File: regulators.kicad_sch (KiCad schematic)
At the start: 47 parts, among them J6 Screw_Terminal_01x02, J7 Screw_Terminal_01x02, SW2 SKRPANE010, U1 STM32H723ZGT6, U7 AP62300TWU, U8 AP2112K-3.3, Y3 25 MHz

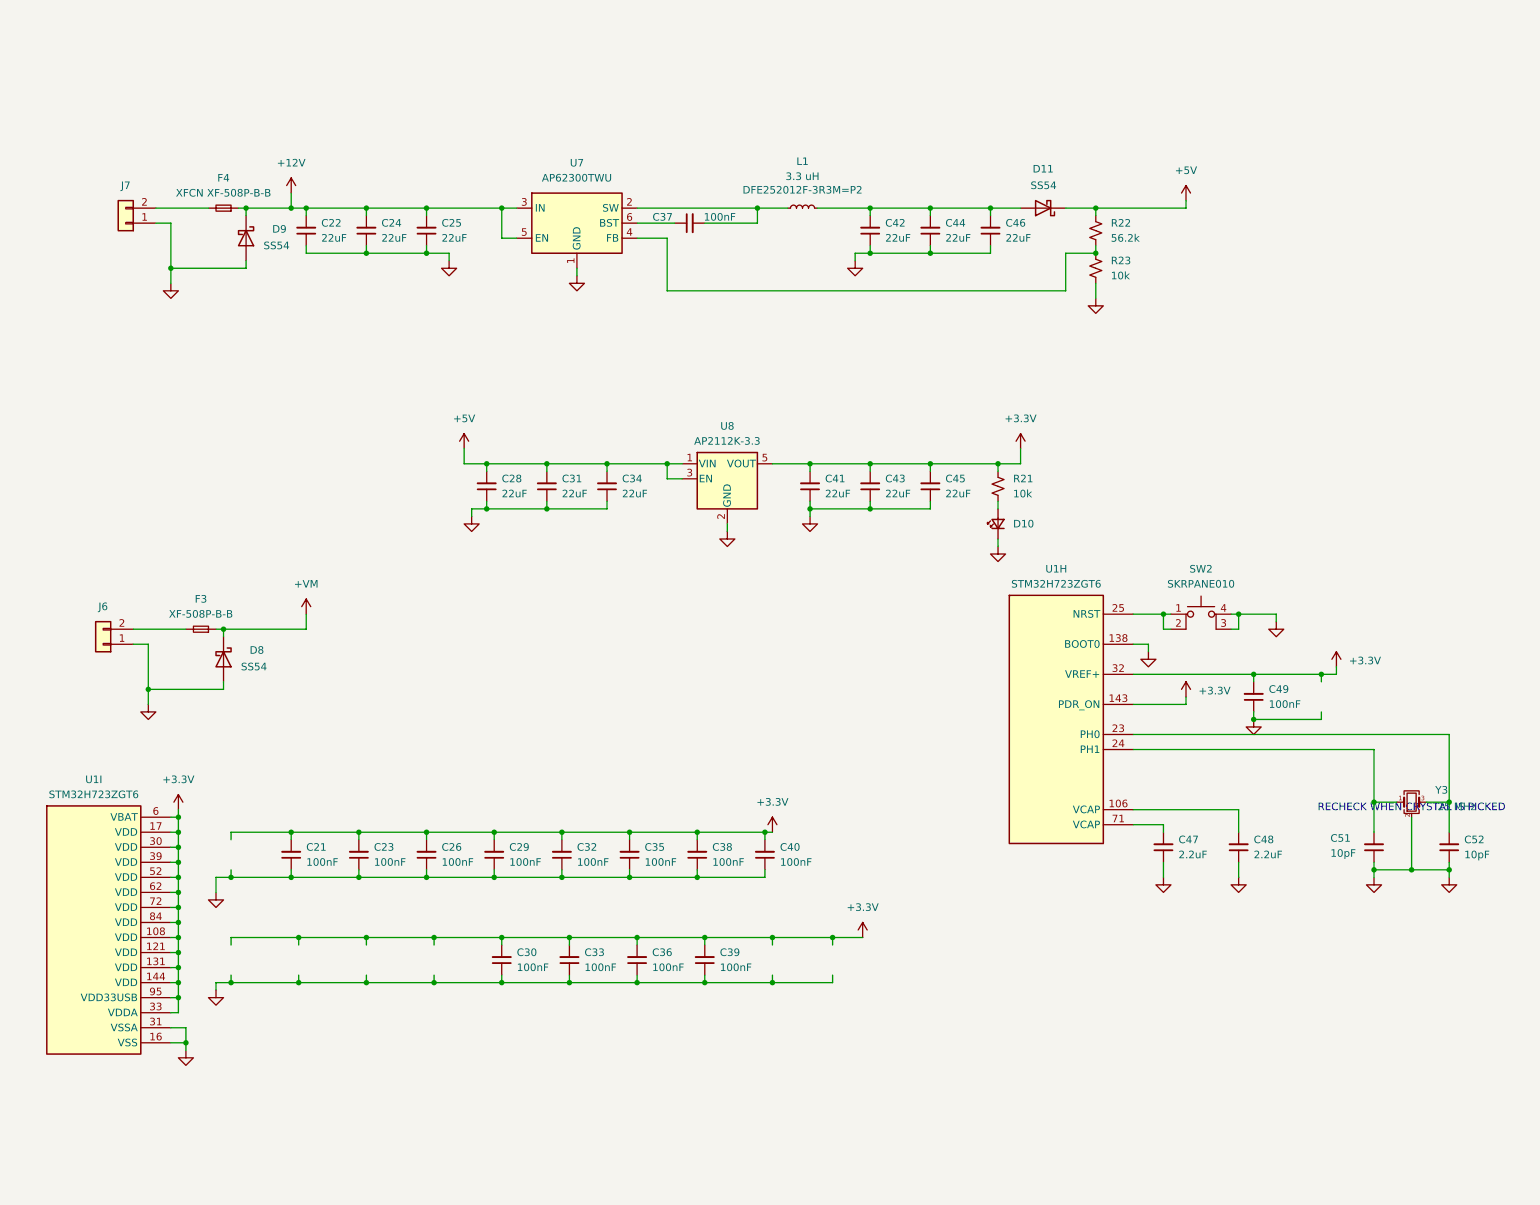
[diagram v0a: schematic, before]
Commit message: ???
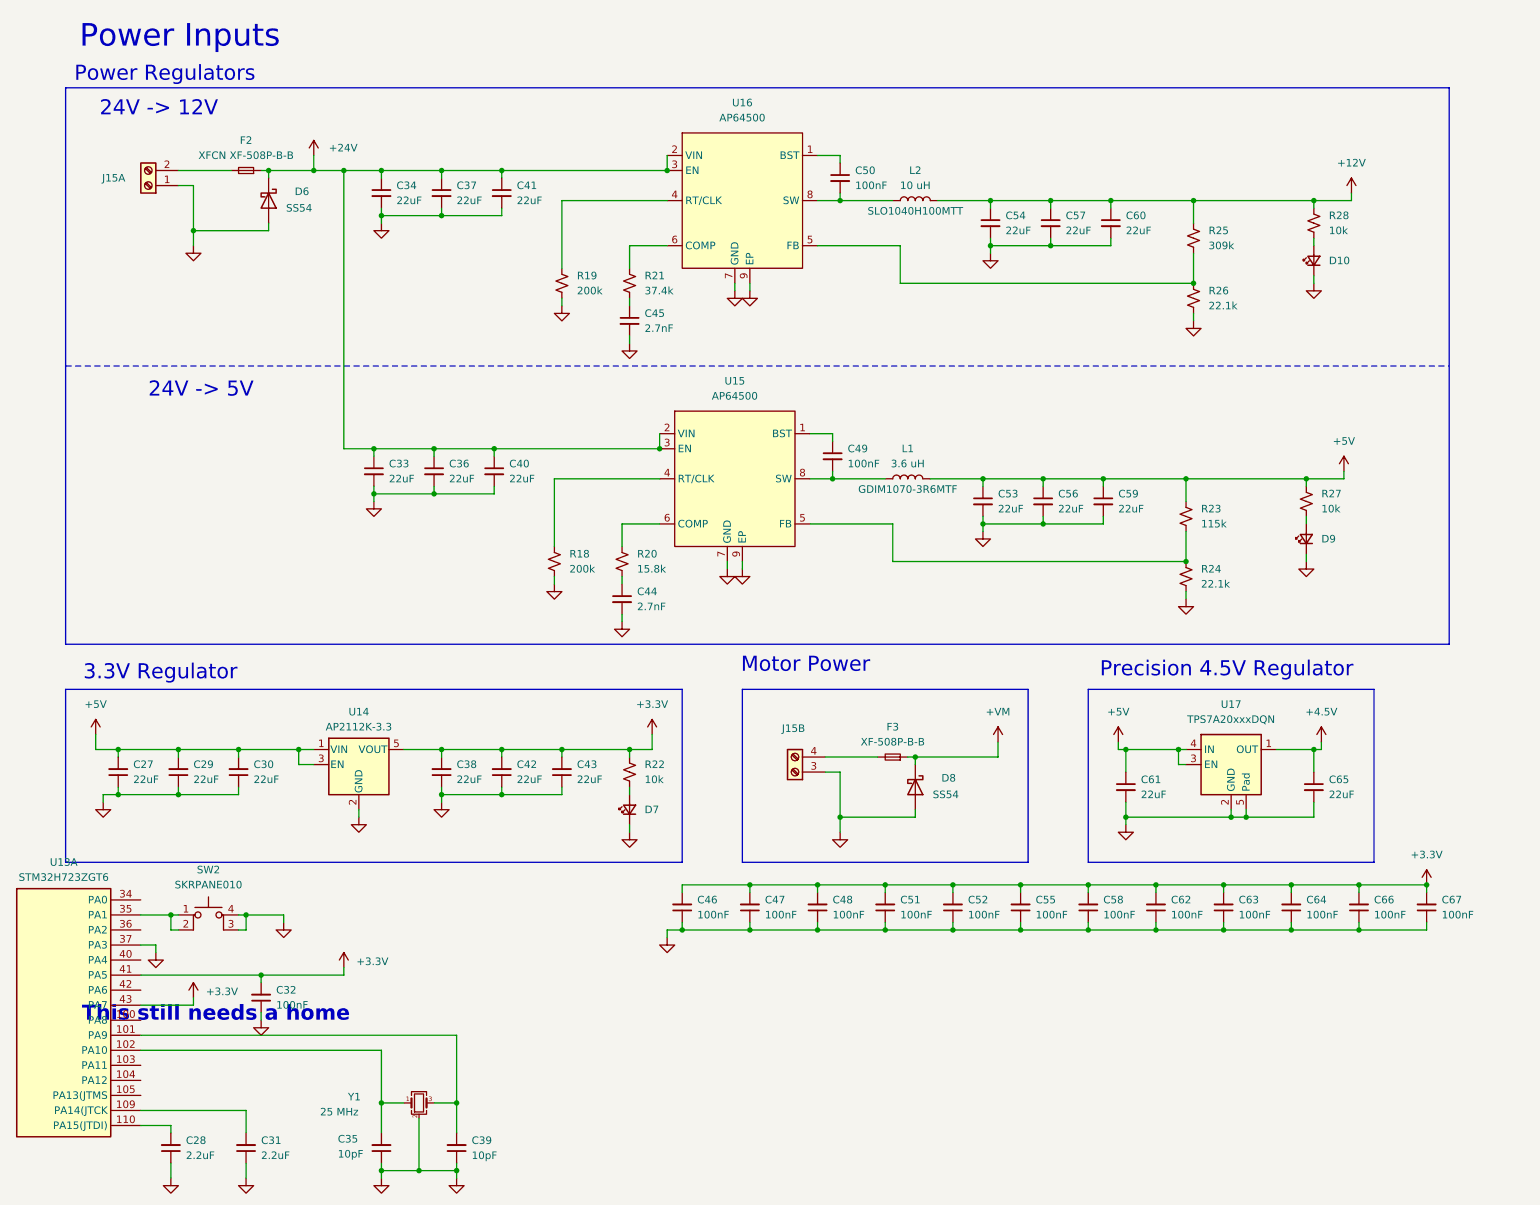
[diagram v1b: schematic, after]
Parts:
- removed C21, C23, C26: 100nF, APRLPrints:C_0603, symbol Device:C_Small
- removed C22, C24, C25: 22uF, APRLPrints:C_0805, symbol Device:C_Small
- removed D11, D9: SS54, Diode_SMD:D_SMA, symbol Diode:SS38
- removed F4: XFCN XF-508P-B-B, Fuse:Fuseholder_Blade_Mini_Keystone_3568, symbol Device:Fuse_Small
- removed J6, J7: Screw_Terminal_01x02, Connector_Phoenix_MSTB:PhoenixContact_MSTBA_2,5_2-G_1x02_P5.00mm_Horizontal, symbol Connector_Generic:Conn_01x02
- removed L1: 3.3 uH, Inductor_SMD:L_1008_2520Metric, symbol Device:L_Small
- removed U1: STM32H723ZGT6, Package_QFP:LQFP-144_20x20mm_P0.5mm, symbol libserie:STM32H723ZGTx
- removed U7: AP62300TWU, Package_TO_SOT_SMD:TSOT-23-6, symbol Regulator_Switching:AP62300TWU
- removed U8: AP2112K-3.3, Package_TO_SOT_SMD:SOT-23-5, symbol Regulator_Linear:AP2112K-3.3
- added C27: 22uF, APRLPrints:C_0805, symbol Device:C_Small
- added C50: 100nF, symbol Device:C_Small
- added C53, C54, C56, C57, C59, C60, C61, C65: 22uF, symbol Device:C_Small
- added C55, C58, C62, C63, C64, C66, C67: 100nF, APRLPrints:C_0603, symbol Device:C_Small
- added D6: SS54, Diode_SMD:D_SMA, symbol Diode:SS38
- added D7, D9: LED_Small, APRLPrints:LED_0603, symbol Device:LED_Small
- added F2: XFCN XF-508P-B-B, Fuse:Fuseholder_Blade_Mini_Keystone_3568, symbol Device:Fuse_Small
- added J15: Screw_Terminal_06x01x02, TerminalBlock_Ningbo-Kagnex:TerminalBlock_Ningbo-Kagnex_HB9500M_1x12_P9.5mm, symbol libserie:Screw_Terminal_06x01x02
- added L1: 3.6 uH, symbol Device:L
- added L2: 10 uH, symbol Device:L
- added R18, R19: 200k, symbol Device:R_Small_US
- added R20: 15.8k, symbol Device:R_Small_US
- added R24, R26: 22.1k, symbol Device:R_Small_US
- added R25: 309k, symbol Device:R_Small_US
- added R27, R28: 10k, APRLPrints:R_0603, symbol Device:R_Small_US
- added U13: STM32H723ZGT6, Package_QFP:LQFP-144_20x20mm_P0.5mm, symbol libserie:STM32H723ZGTx
- added U14: AP2112K-3.3, Package_TO_SOT_SMD:SOT-23-5, symbol Regulator_Linear:AP2112K-3.3
- added U15, U16: AP64500, Package_SO:Diodes_SO-8EP, symbol libserie:AP64500-EP
- added U17: TPS7A20xxxDQN, Package_SON:Texas_X2SON-4_1x1mm_P0.65mm, symbol Regulator_Linear:TPS7A20xxxDQN
- C28, C31: value 22uF -> 2.2uF; footprint APRLPrints:C_0805 -> APRLPrints:C_0603
- C29, C30, C38: value 100nF -> 22uF; footprint APRLPrints:C_0603 -> APRLPrints:C_0805
- C33, C36, C37, C40: value 100nF -> 22uF; footprint APRLPrints:C_0603 -> (none)
- C34, C41: footprint APRLPrints:C_0805 -> (none)
- C35, C39: value 100nF -> 10pF
- C44, C45: value 22uF -> 2.7nF; footprint APRLPrints:C_0805 -> (none)
- C46: value 22uF -> 100nF; footprint APRLPrints:C_0805 -> APRLPrints:C_0603
- C47, C48: value 2.2uF -> 100nF
- C49: footprint APRLPrints:C_0603 -> (none)
- C51, C52: value 10pF -> 100nF
- R21: value 10k -> 37.4k; footprint APRLPrints:R_0603 -> (none)
- R22: value 56.2k -> 10k
- R23: value 10k -> 115k; footprint APRLPrints:R_0603 -> (none)
- Y1: renamed from Y3; private (none) -> KLC_S4.1
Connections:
- net +12V: now also C54.1, C57.1, C60.1, L2.2, R25.1, R28.1
- net +3.3V: now also C42.2, C46.2, C47.2, C48.2, C51.2, C52.2, R22.1, C55.2, C58.2, C62.2, C63.2, C64.2, C66.2, C67.2, U13.41 (PA5), U13.43 (PA7), U14.5 (VOUT); no longer C29.2, C30.2, C33.2, C35.2, C36.2, C39.2, C40.2, C41.2, C45.2, C49.2, R21.1
- net +5V: now also C29.2, C30.2, R23.1, C27.2, C53.1, C56.1, C59.1, C61.1, L1.2, R27.1, U14.1 (VIN), U14.3 (EN), U17.3 (EN), U17.4 (IN); no longer C28.2, C31.2, C34.2, R22.1
- net GND: now also C33.2, C34.2, C36.2, C37.2, C40.2, C41.2, C44.2, C45.2, C27.1, C53.2, C54.2, C55.1, C56.2, C57.2, C58.1, C59.2, C60.2, C61.2, C62.1, C63.1, C64.1, C65.2, C66.1, C67.1, D6.2 (A), D7.1 (K), D9.1 (K), J15.1 (Pin_1), J15.3 (Pin_1), R18.2, R19.2, R24.2, R26.2, U13.37 (PA3), U14.2 (GND), U15.7 (GND), U15.9 (EP), U16.7 (GND), U16.9 (EP), U17.2 (GND), U17.5 (Pad); no longer C33.1, C34.1, C36.1, C40.1, C41.1, C44.1, C45.1, C49.1, R23.2
- net at R22.2: now also D7.2 (A); no longer R23.1
- net at F3.2: now also J15.4 (Pin_2)
- net at Y1.1: now also C35.2, U13.102 (PA10); no longer C51.2
- net +24V: now reaches C37.1
- net +24V: now also C33.1, C34.1, C36.1, C40.1, C41.1, D6.1 (K), F2.1, U15.2 (VIN), U15.3 (EN), U16.2 (VIN), U16.3 (EN)
- net at SW2.1, SW2.2: now also U13.35 (PA1)
- net at Y1.3: now also C39.2, U13.101 (PA9); no longer C52.2
- net at R21.2: now also C45.1; no longer D10.2 (A)
- new net: C49.2, L1.1, U15.8 (SW)
- new net: R23.2, R24.1, U15.5 (FB)
- new net: D10.2 (A), R28.2
- new net: D9.2 (A), R27.2
- new net: C49.1, U15.1 (BST)
- new net: R18.1, U15.4 (RT/CLK)
- new net: R20.1, U15.6 (COMP)
- new net: C44.1, R20.2
- new net: C31.2, U13.109 (PA14(JTCK)
- new net: C28.2, U13.110 (PA15(JTDI))
- new net: R19.1, U16.4 (RT/CLK)
- new net: R21.1, U16.6 (COMP)
- new net: F2.2, J15.2 (Pin_2)
- new net: R25.2, R26.1, U16.5 (FB)
- new net: C50.1, U16.1 (BST)
- new net: C50.2, L2.1, U16.8 (SW)
- new net +4.5V: C65.1, U17.1 (OUT)
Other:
- note added: "24V -> 12V"
- note added: "24V -> 5V"
- note added: "3.3V Regulator"
- note added: "Motor Power"
- note added: "Power Inputs"
- note added: "Power Regulators"
- note added: "Precision 4.5V Regulator"
- note added: "This still needs a home"
- note removed: "RECHECK WHEN CRYSTAL IS PICKED"
- moved on the sheet: SW2, Y1
